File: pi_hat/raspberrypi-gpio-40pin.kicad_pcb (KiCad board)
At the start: 2 copper layers, 86.8 x 69.4 mm, 82 parts, among them J1 MC000052, J2 10pinIDC, J3 MOLEX_2031, P1 Conn_02x20_Odd_Even, Q1 IRLB8721PBF, SW1 SW_Push, U1 iCE40-HX4K-TQ144, U2 MCP1826S-3302E/DB, U3 MCP1826S-1202E/DB, U4 S25FL064LABMFI010, Y1 SIT8008BI-12-XXE-100

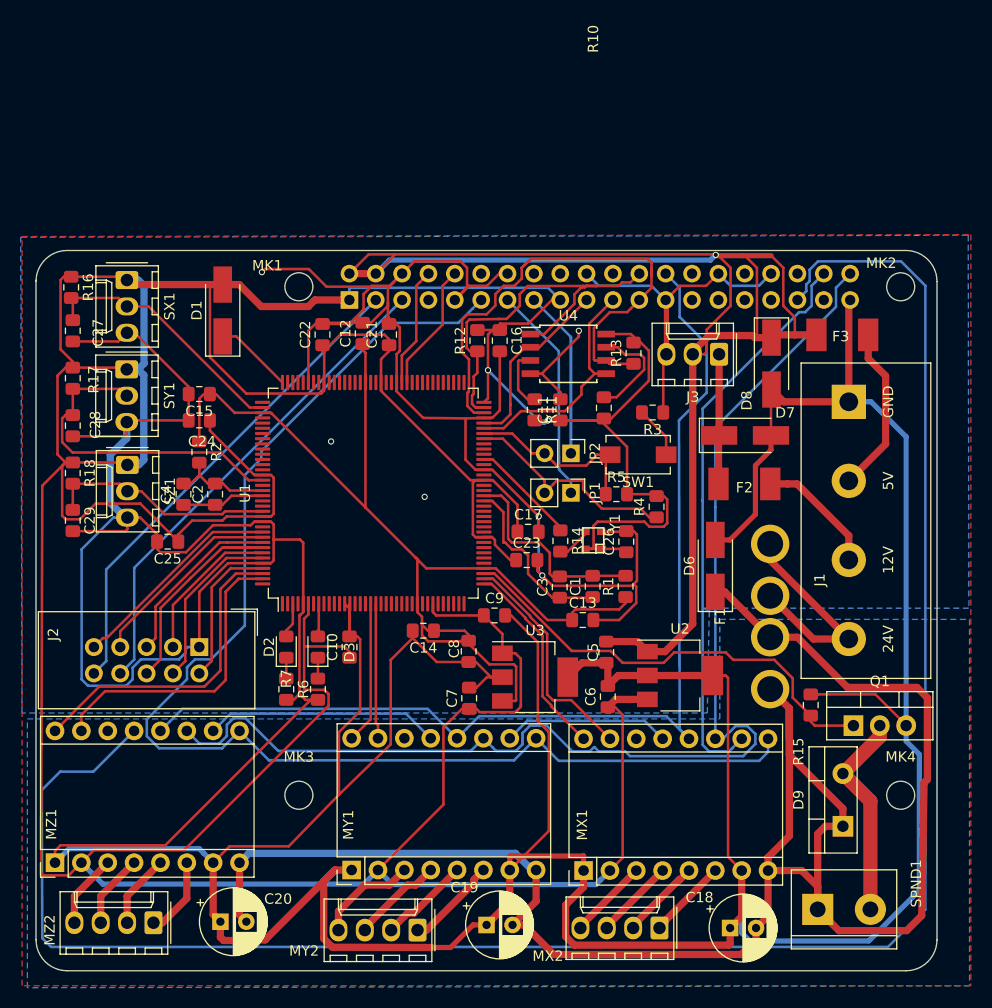
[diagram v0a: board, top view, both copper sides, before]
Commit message: finished routing
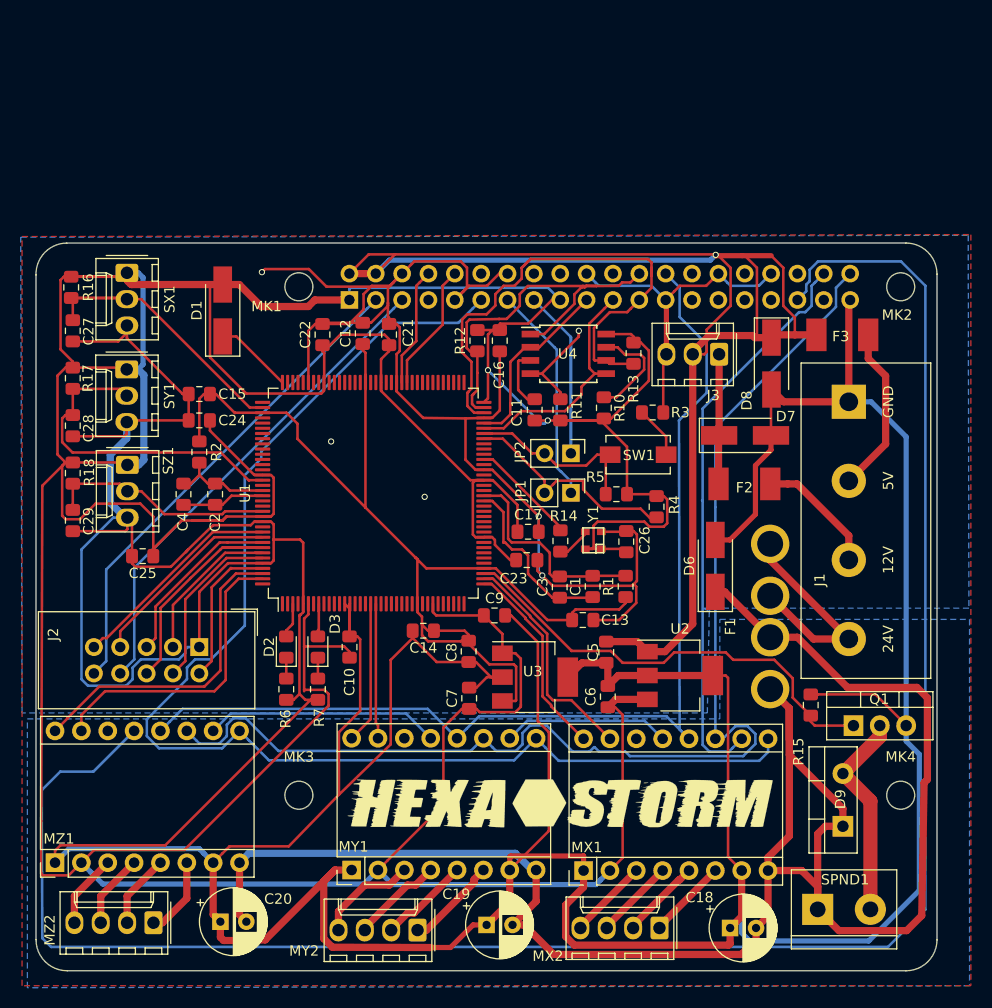
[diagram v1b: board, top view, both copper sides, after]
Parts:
- added G1: hexastorm, footprints:hexastorm, F.Cu at (228.6, 147.3)
- moved C25 2.79 mm to (188.4, 123.5)
- moved SX1 0.70 mm to (186.9, 96.2)
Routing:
- net +3V3: track 504.8 -> 528.0 mm
- net X_PO: track 25.0 -> 30.7 mm
- net GND: track 709.8 -> 713.4 mm
- net +1V2: track 100.3 -> 101.2 mm
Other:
- board size 86.8 x 69.4 mm -> 86.8 x 70.1 mm
